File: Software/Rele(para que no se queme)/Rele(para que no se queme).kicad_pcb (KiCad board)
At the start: 2 copper layers, 100 x 100.1 mm, 56 parts, among them J1 Screw_Terminal_01x02, J10 Screw_Terminal_01x02, J11 Screw_Terminal_01x02, J2 Screw_Terminal_01x02, J3 Screw_Terminal_01x02, J4 Screw_Terminal_01x02, J5 Screw_Terminal_01x04, J6 Screw_Terminal_01x02, J7 Screw_Terminal_01x02, J9 Screw_Terminal_01x02, K1 G5V-2, K2 G5V-2, K4 G5V-2, K5 G5V-2, Q1 BC547, Q2 BC547, Q5 BC547, U1 PC817, U2 PC817, U3 PC817, U4 L7805, U5 ESP32_DEVKITC, U6 PC817

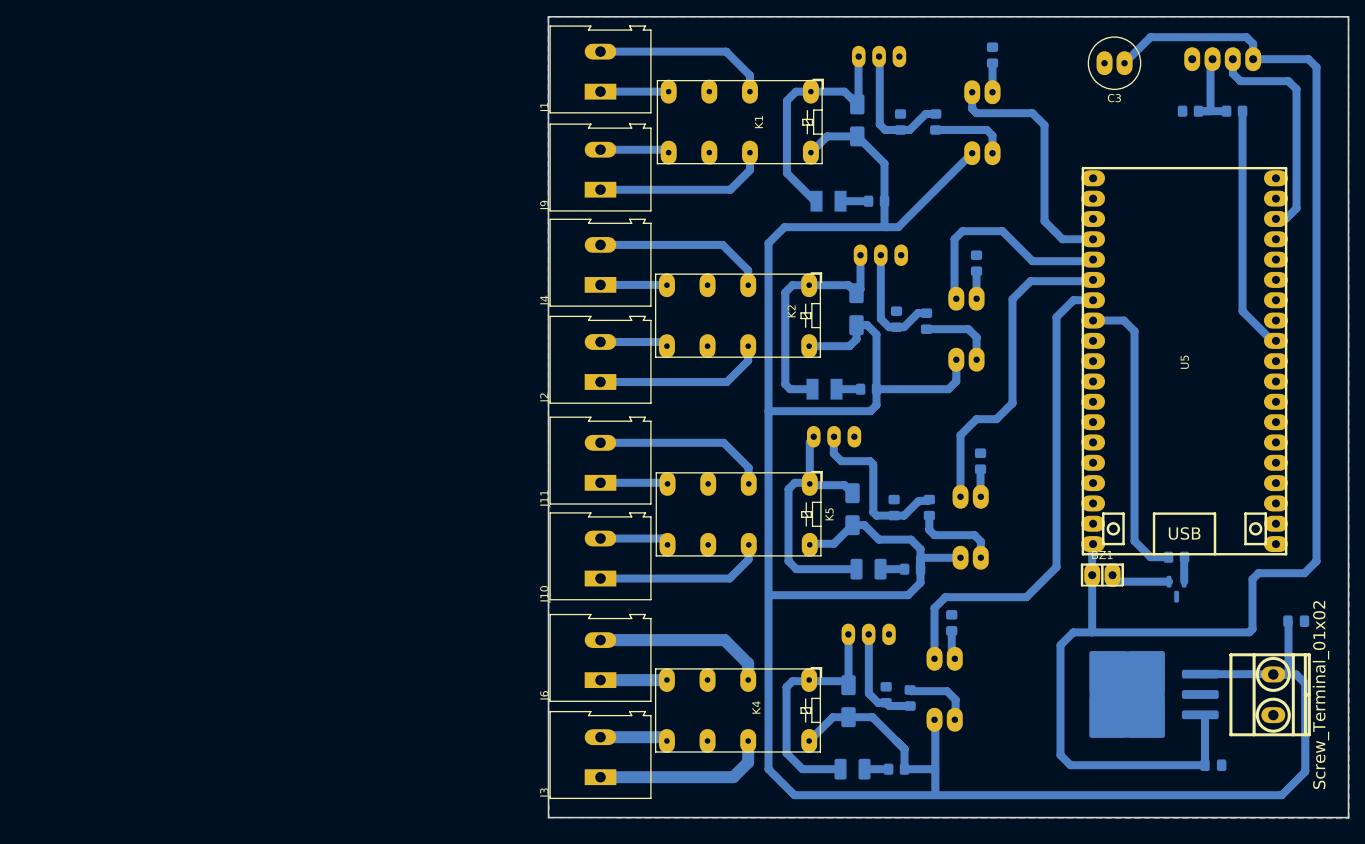
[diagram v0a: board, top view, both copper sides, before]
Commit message: Add files via upload
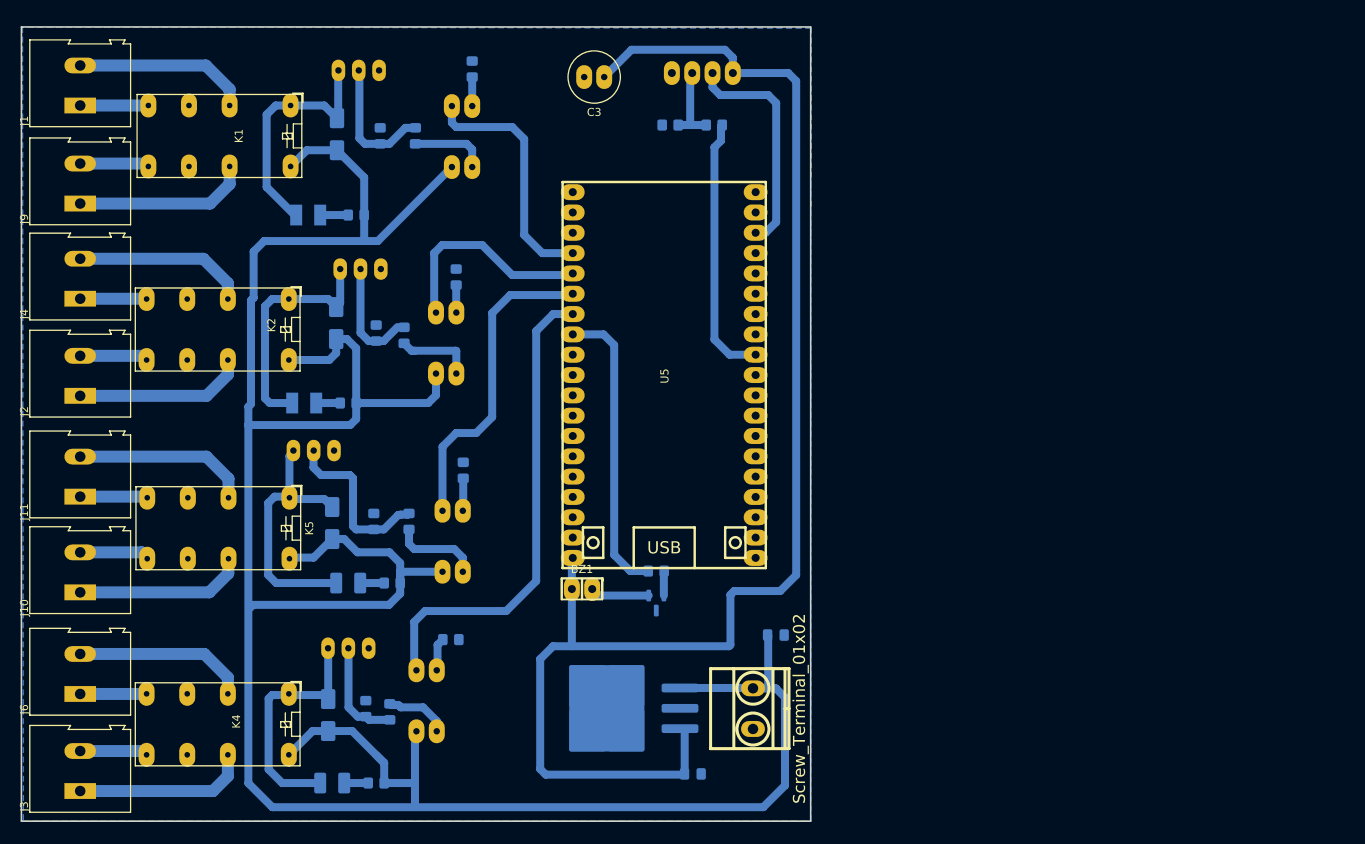
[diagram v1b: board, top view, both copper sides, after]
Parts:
- moved R5 65.3 mm to (79.9, 89.3)
- moved C2 65.1 mm to (116.0, 144.1)
- moved C1 65.1 mm to (126.4, 126.7)
- moved C3 65.1 mm to (105.0, 57.0)
- moved D2 65.1 mm to (71.5, 87.7)
- moved D3 65.1 mm to (70.5, 136.7)
- moved D4 65.1 mm to (71.0, 112.7)
- moved D5 65.1 mm to (68.0, 74.2)
- moved D6 65.1 mm to (71.0, 145.2)
- moved D7 65.1 mm to (67.5, 97.7)
- moved D8 65.1 mm to (73.0, 120.2)
- moved J5 65.1 mm to (117.2, 56.5)
- moved K1 65.1 mm to (65.8, 60.5)
- moved K2 65.1 mm to (65.5, 84.7)
- moved K4 65.1 mm to (65.5, 134.1)
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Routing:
- net trig: track 30.7 -> 33.1 mm
- net Net-(Q2-B): track 14.8 -> 13.8 mm
- net Net-(R7-Pad2): track 3.40 -> 4.10 mm
- net +5V: track 178.9 -> 178.3 mm
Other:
- board size 100 x 100.1 mm -> 98.7 x 99.3 mm
